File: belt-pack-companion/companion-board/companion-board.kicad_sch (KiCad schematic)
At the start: 34 parts, among them J1 Conn_01x18_Socket, J2 Conn_01x18_Socket, J3 AudioJack4_Ground, J4 Micro_SD_Card, U1 TLV320AIC3204

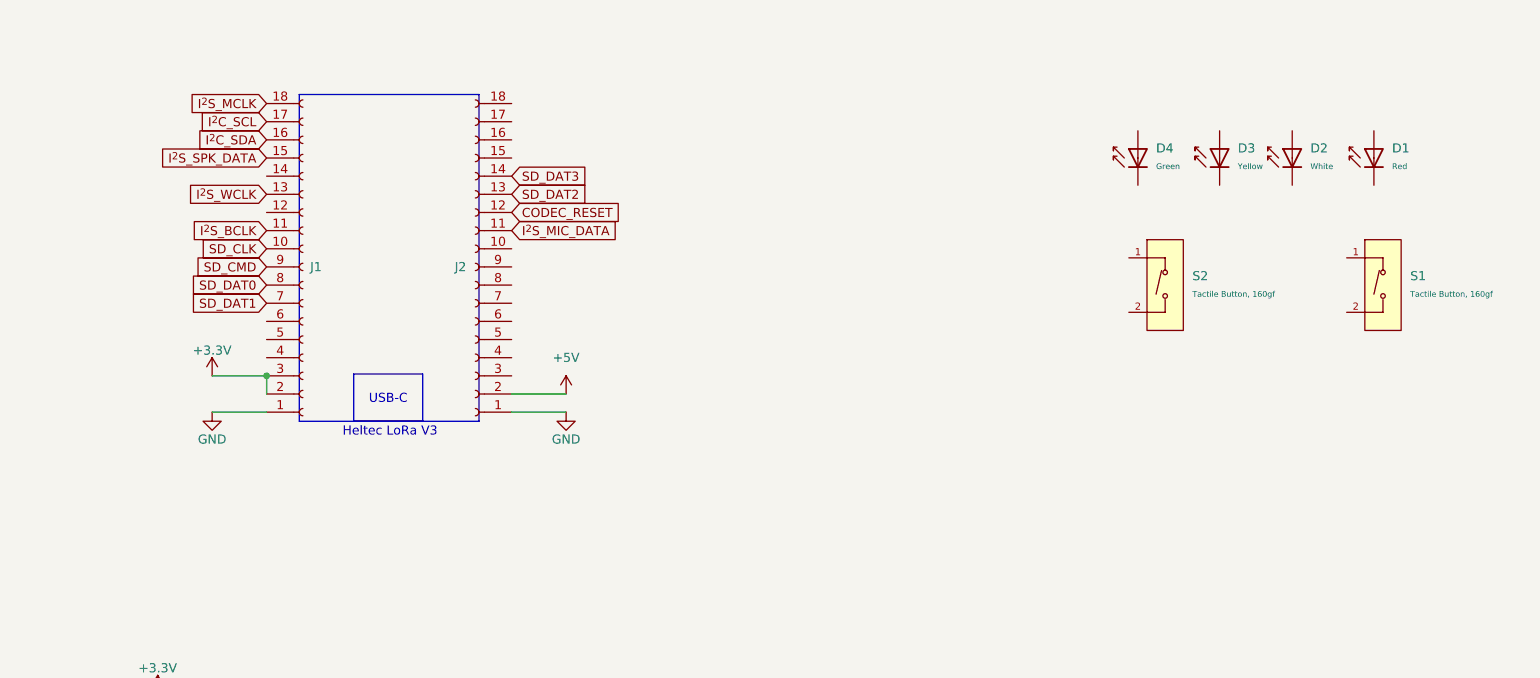
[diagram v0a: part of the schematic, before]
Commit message: Schematic Progress
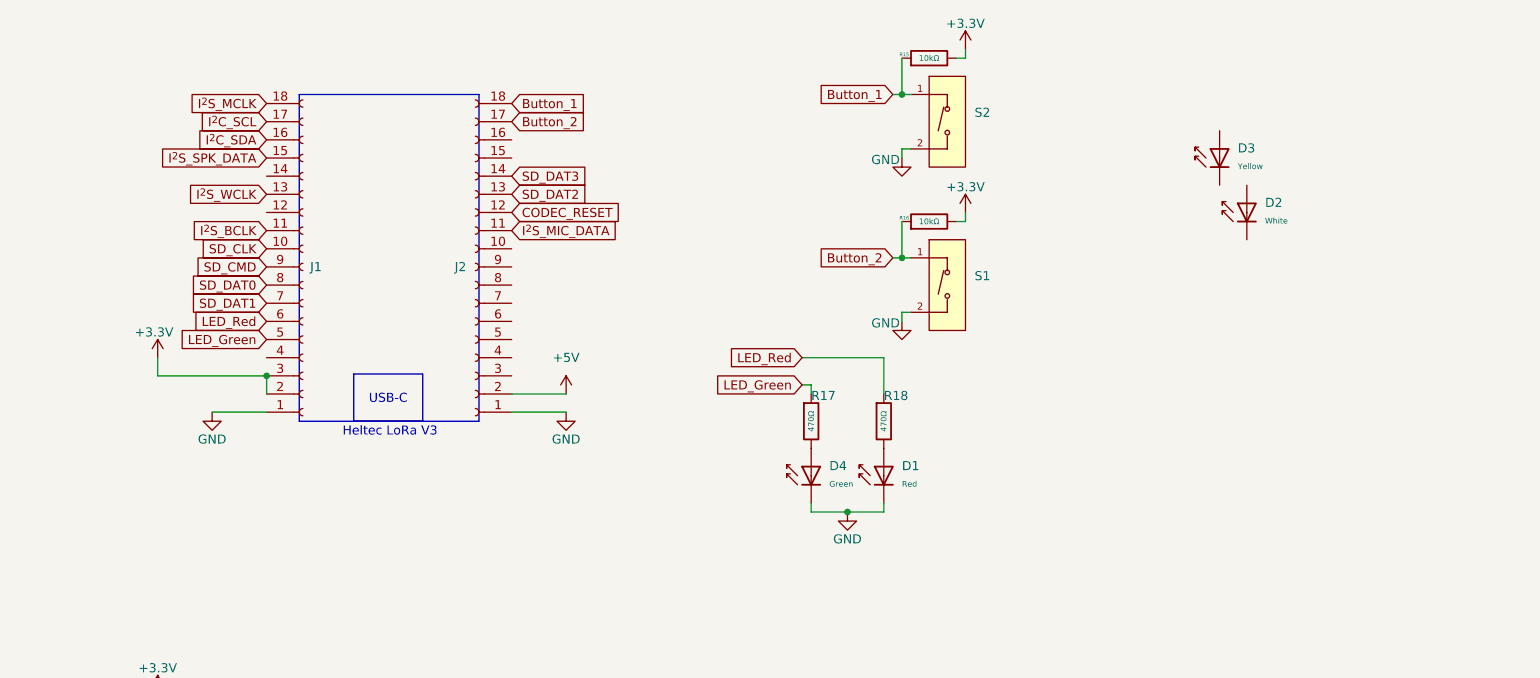
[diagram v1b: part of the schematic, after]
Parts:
- added R15, R16: 10kΩ, PCM_JLCPCB:R_0402, symbol PCM_JLCPCB-Resistors:0402,10kΩ
- added R17, R18: 470Ω, PCM_JLCPCB:R_0402, symbol PCM_JLCPCB-Resistors:0402,470Ω
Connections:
- net +3.3V: now also R15.2, R16.2
- net GND: now also D1.1, D4.1, S1.2 (B), S2.2 (B)
- net Button_2: now reaches J2.17 (Pin_17)
- net Button_2: now also S1.1 (A), R16.1
- net Button_1: now reaches J2.18 (Pin_18)
- net Button_1: now also S2.1 (A), R15.1
- net at D4.2: now also R17.2
- net at D1.2: now also R18.2
- net LED_Green: now reaches J1.5 (Pin_5)
- net LED_Green: now also R17.1
- net LED_Red: now reaches J1.6 (Pin_6)
- net LED_Red: now also R18.1
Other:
- moved on the sheet: D1, D2, D4, S1, S2
